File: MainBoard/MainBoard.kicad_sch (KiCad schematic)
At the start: 30 parts, among them J1 1761681-3, Q1 BC557, Q2 BC557, Q3 BC557, Q4 BC557, Q5 BC547, Q6 BC547, Q7 BC547, Q8 BC547

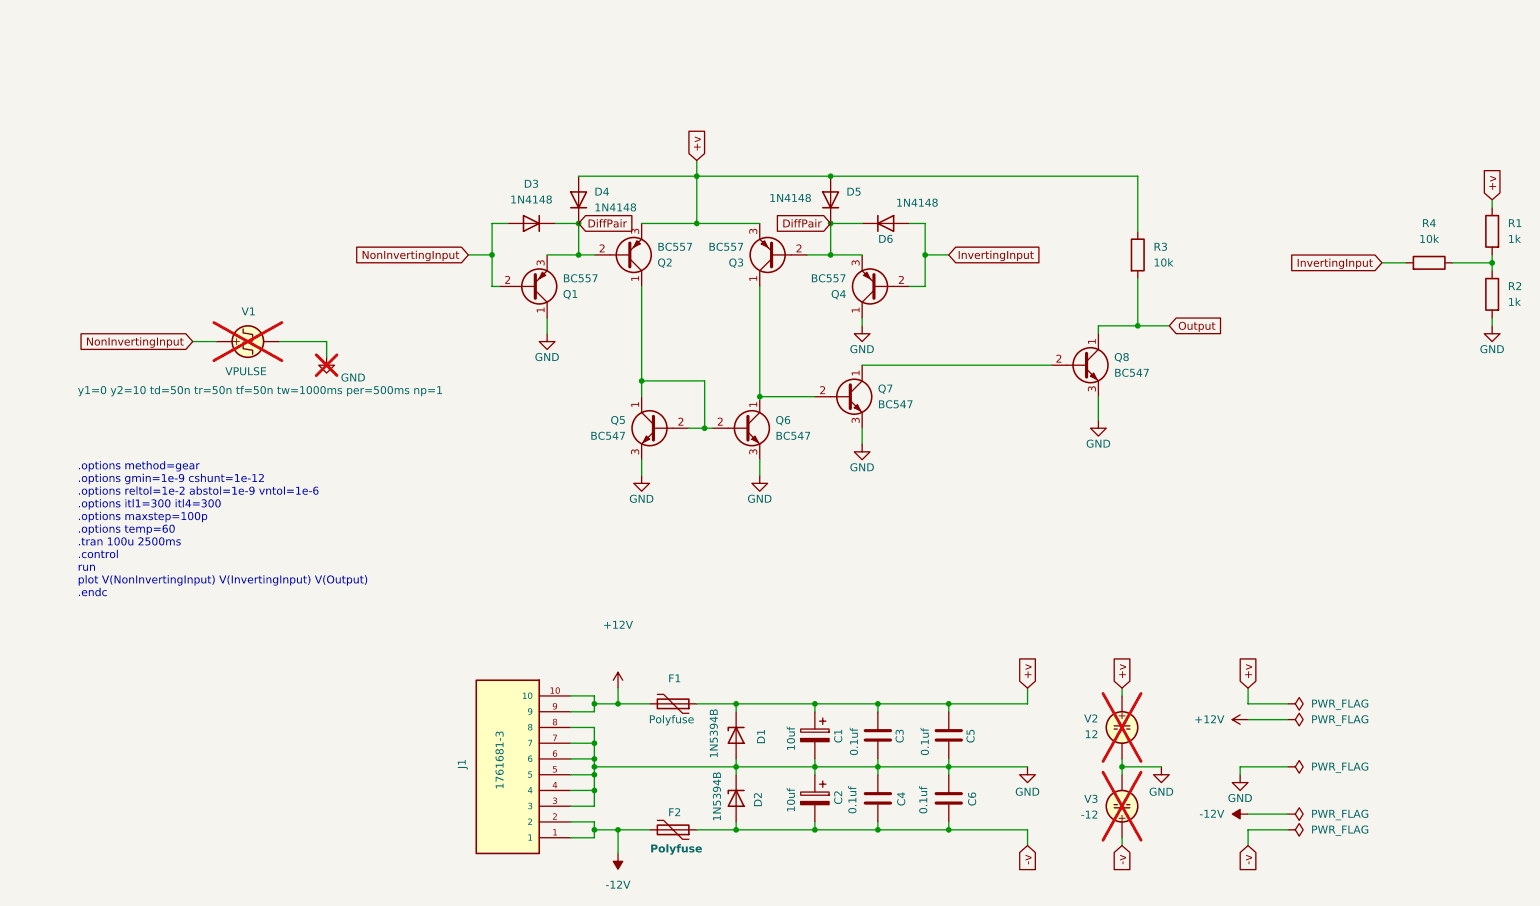
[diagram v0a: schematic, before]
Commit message: snapshot
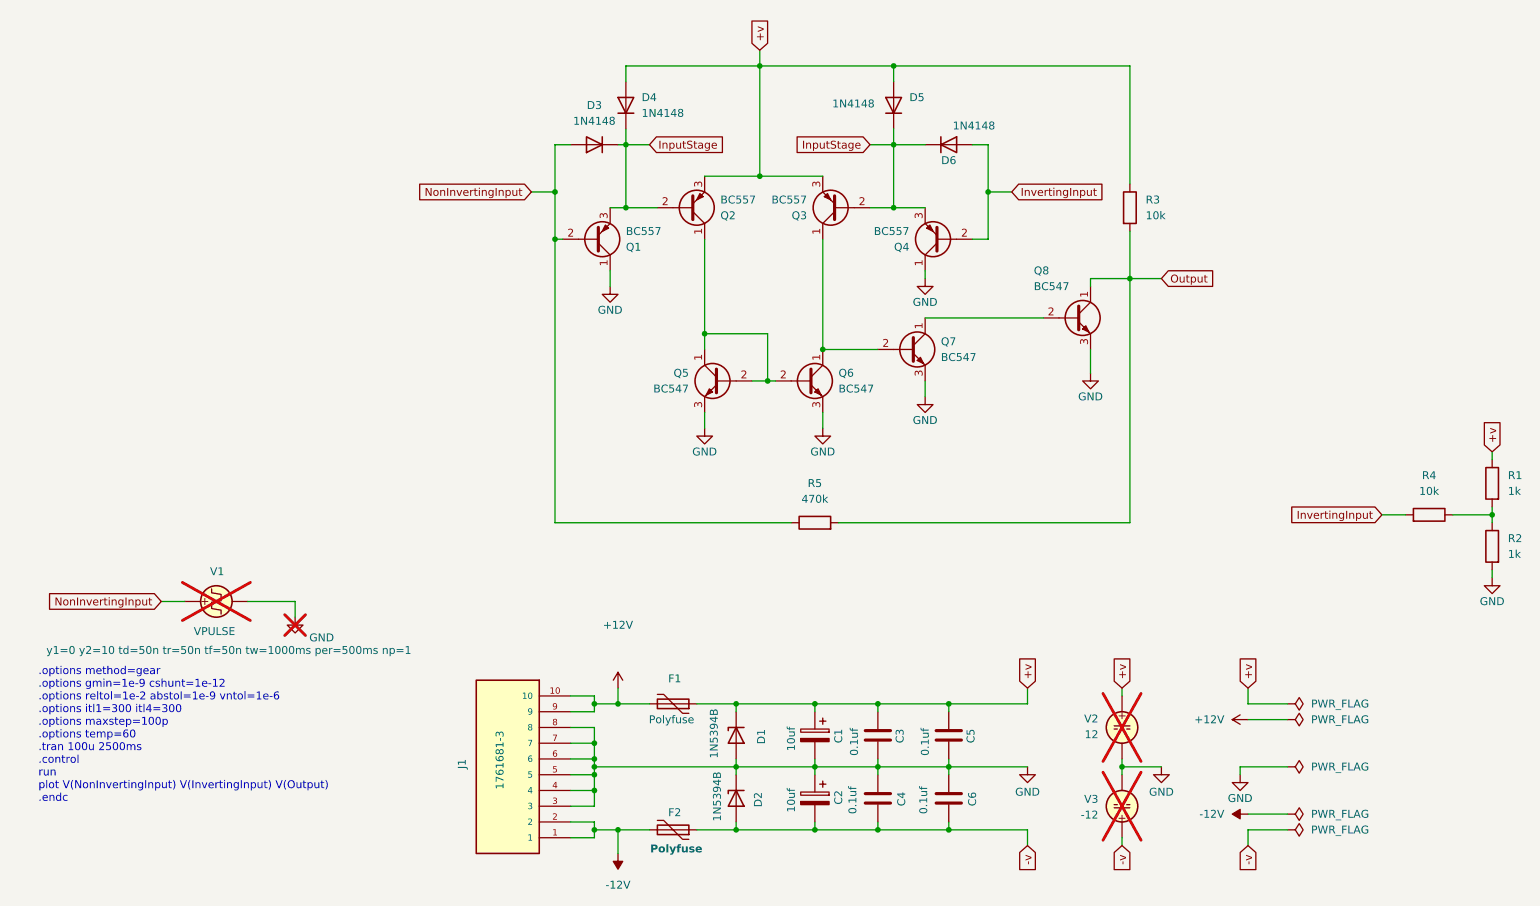
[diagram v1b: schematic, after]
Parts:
- added R5: 470k, symbol Device:R
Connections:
- net NonInvertingInput: now also R5.1
- net Output: now also R5.2
- net DiffPair renamed InputStage
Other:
- moved on the sheet: D3, D4, D5, D6, Q1, Q2, Q3, Q4, Q5, Q6, Q7, Q8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
